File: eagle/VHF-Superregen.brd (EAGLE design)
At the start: 33 x 30.5 mm, 22 parts, among them SW1 SL-SW-1P-2T-H, T1 2N3904

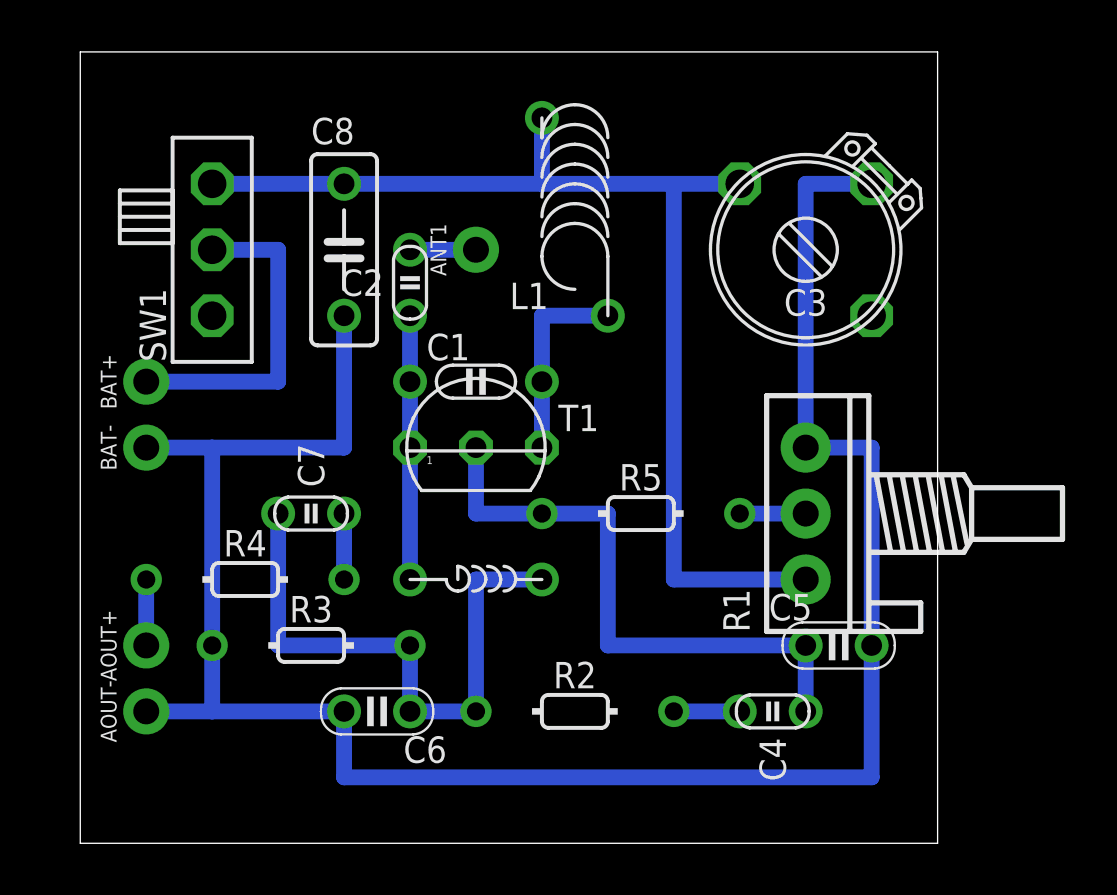
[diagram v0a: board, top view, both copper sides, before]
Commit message: ...
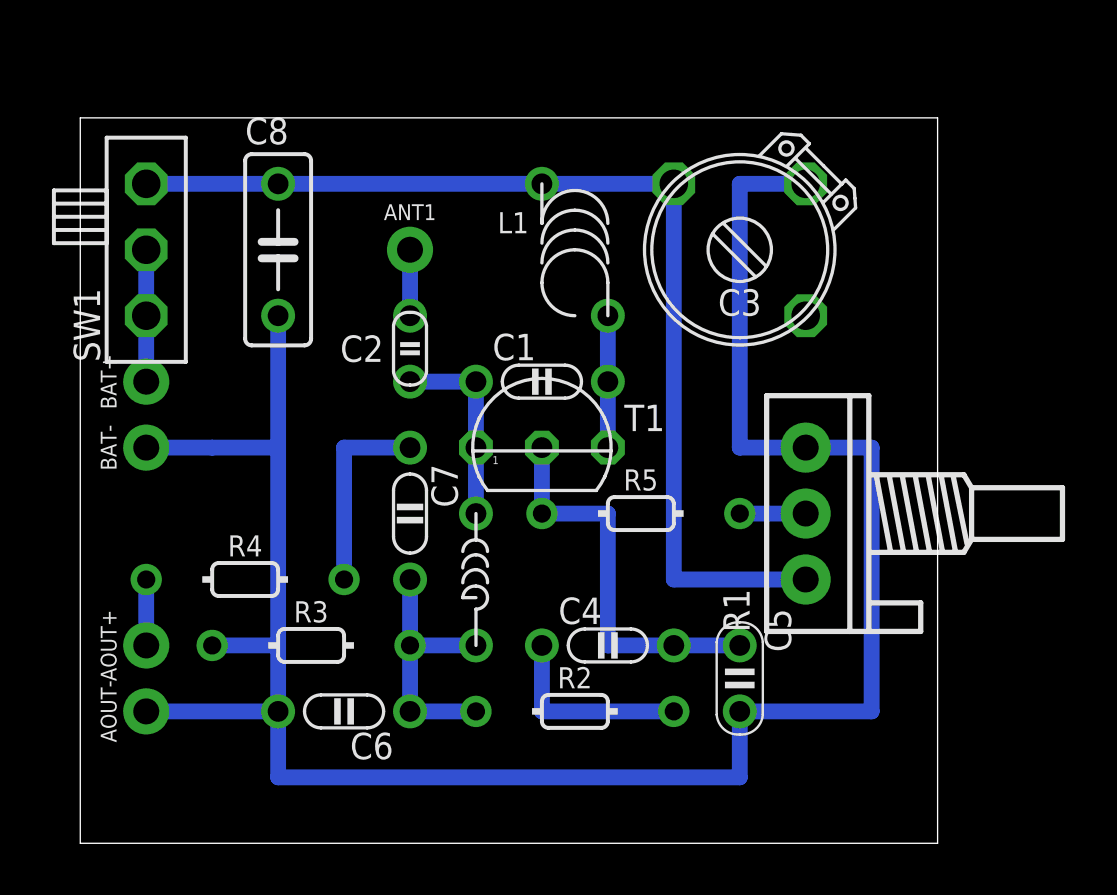
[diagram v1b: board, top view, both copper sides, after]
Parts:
- C4, C7: device c:C025-015X024 -> c:C050-020X036
- C6: device c:C025-020X036 -> c:C050-020X036
- L1: device r:L-04/7V -> l:L-04-5/5V
- moved C4 6.84 mm to (20.3, 7.62), turned to 0 degrees
- moved C7 3.81 mm to (12.7, 12.7)
- moved C3 2.54 mm to (25.4, 22.9)
- moved C5 2.54 mm to (25.4, 7.62), turned to 270 degrees
- moved ANT1 2.54 mm to (12.7, 22.9), turned to 270 degrees
- moved C1 2.54 mm to (17.8, 17.8)
- moved T1 2.54 mm to (17.8, 15.2)
- moved C8 2.54 mm to (7.62, 22.9)
- moved SW1 2.54 mm to (2.54, 22.9)
- moved C2 2.54 mm to (12.7, 19.1)
- moved C6 2.54 mm to (10.2, 5.08)
- moved L1 2.54 mm to (19.1, 22.9)
- turned L2 to 0 degrees
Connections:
- net N$1: now also L1.2; no longer L1.1
- net N$12: now also L2.2; no longer L2.1
- net N$2: now also L2.1; no longer L2.2
- net N$3: now also L1.1; no longer L1.2
- net N$9: now also SW1.3
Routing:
- net N$12: track 22.9 -> 10.2 mm
- net N$4: track 22.9 -> 15.2 mm
- net N$9: track 12.7 -> 5.08 mm
- net N$8: track 2.54 -> 7.62 mm
- net N$7: track 2.54 -> 7.62 mm
- net GND: track 81.3 -> 83.8 mm
- net N$3: track 43.2 -> 40.6 mm
- net N$1: track 7.62 -> 5.08 mm
- net N$2: track 10.2 -> 7.62 mm
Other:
- board size 33 x 30.5 mm -> 33 x 27.9 mm
